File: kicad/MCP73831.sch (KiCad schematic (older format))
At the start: 13 parts, among them J1 BATT, U2 MCP73831-2

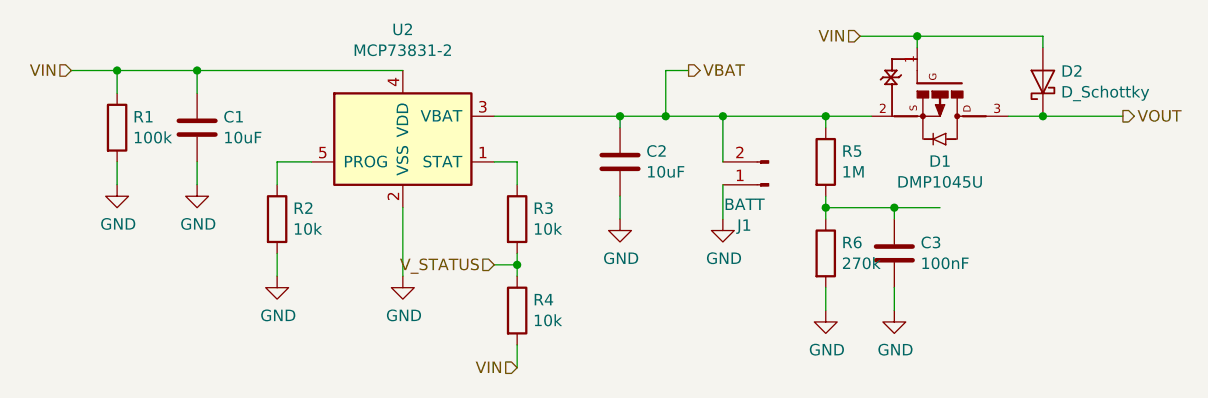
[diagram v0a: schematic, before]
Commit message: working on routing
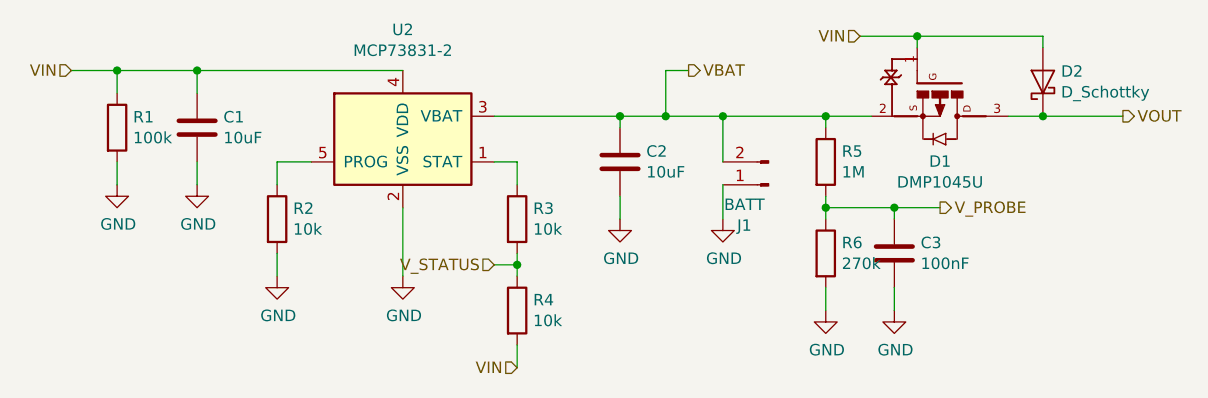
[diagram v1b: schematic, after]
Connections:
- net V_PROBE: now reaches C3.1, R5.2, R6.1
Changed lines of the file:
@@
 Wire Wire Line
 	6850 2700 7100 2700
+Text HLabel 8050 3100 2    50   Output ~ 0
+V_PROBE
 $EndSCHEMATC
